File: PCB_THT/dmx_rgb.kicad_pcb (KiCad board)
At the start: 2 copper layers, 30 parts, among them J1 CONN_01X02, J2 Conn_02x04_Odd_Even, J3 Conn_02x03_Odd_Even, J4 CONN_01X03, J5 CONN_01X04, J6 CONN_01X04, Q1 Q_NMOS_GDS, Q2 Q_NMOS_GDS, Q3 Q_NMOS_GDS, U1 ATTINY2313-20PU, U2 L7805, U3 MAX485E, Y1 Crystal

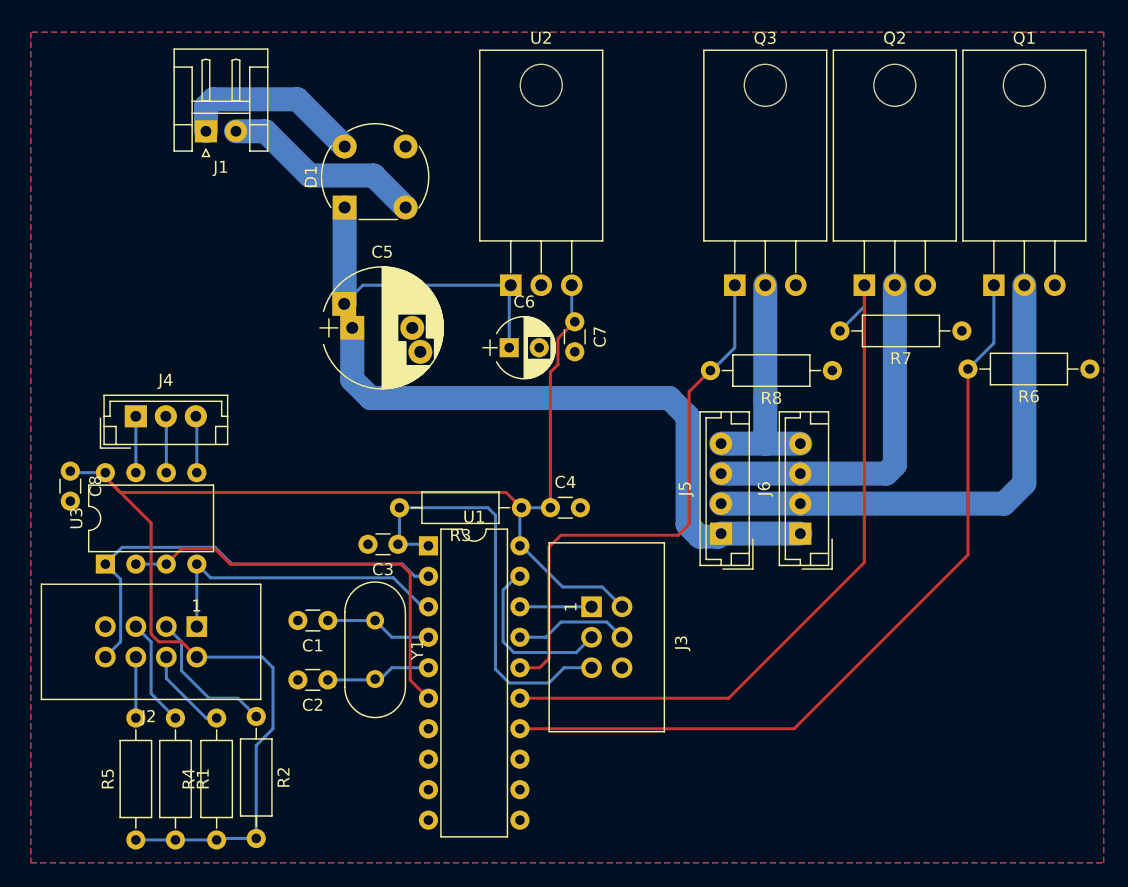
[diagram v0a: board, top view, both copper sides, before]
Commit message: Board geändert
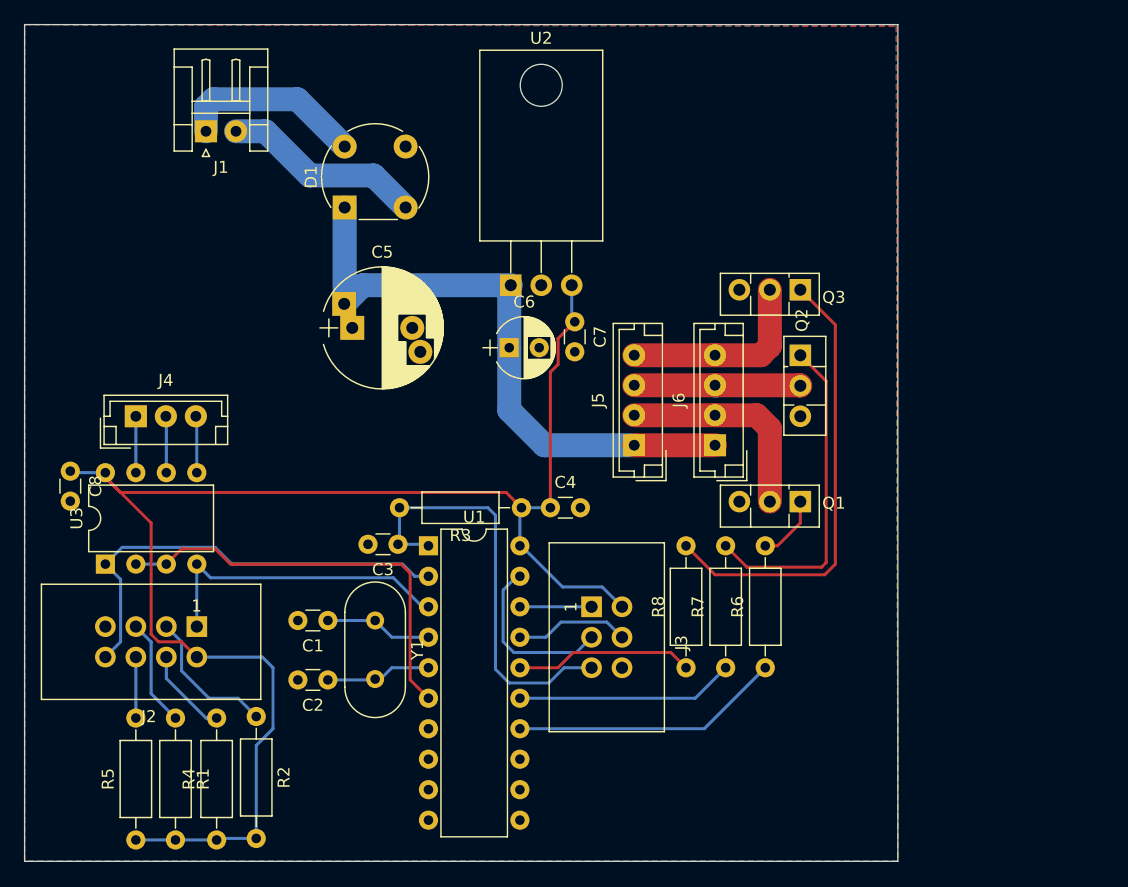
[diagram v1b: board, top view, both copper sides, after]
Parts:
- Q1, Q2, Q3: value Q_NMOS_GDS -> Q_NPN_BCE; footprint TO_SOT_Packages_THT:TO-220_Horizontal -> TO_SOT_Packages_THT:TO-126_Vertical
- moved R6 36.8 mm to (216.0, 117.9), turned to 90 degrees
- moved R7 34.3 mm to (212.7, 117.9), turned to 90 degrees
- moved R8 27.6 mm to (209.4, 117.9), turned to 90 degrees
- moved Q1 24.2 mm to (218.9, 104.0), turned to 180 degrees
- moved J5 10.3 mm to (205.1, 99.3)
- moved J6 10.2 mm to (211.8, 99.3)
- moved Q2 7.91 mm to (218.9, 91.8), turned to 270 degrees
- moved Q3 5.47 mm to (218.9, 86.4), turned to 180 degrees
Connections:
- Q1 pad 1: /PWM1 -> Net-(Q1-Pad1)
- Q2 pad 1: /PWM2 -> Net-(Q2-Pad1)
- Q3 pad 1: /PWM3 -> Net-(Q3-Pad1)
- R6 pad 1: GND -> /PWM1
- R6 pad 2: /PWM1 -> Net-(Q1-Pad1)
- R7 pad 1: GND -> /PWM2
- R7 pad 2: /PWM2 -> Net-(Q2-Pad1)
- R8 pad 1: GND -> /PWM3
- R8 pad 2: /PWM3 -> Net-(Q3-Pad1)
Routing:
- net /PWM1: track 66.7 -> 22.6 mm
- net /PWM2: track 61.1 -> 18.2 mm
- net Net-(Q3-Pad1): track 0.00 -> 37.9 mm
- net /PWM3: track 46.1 -> 14.9 mm
- net +12V: track 80.3 -> 51.4 mm
- net Net-(Q2-Pad1): track 0.00 -> 27.6 mm
- net Net-(J5-Pad2): track 42.5 -> 17.9 mm
- net Net-(J5-Pad3): track 29.8 -> 13.9 mm
- net Net-(Q1-Pad1): track 0.00 -> 5.62 mm
- net Net-(J5-Pad4): track 19.8 -> 16.3 mm
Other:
- board outline added: 72.8 x 69.7 mm
